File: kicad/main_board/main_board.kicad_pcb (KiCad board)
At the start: 2 copper layers, 42 parts, among them J1 Barrel_Jack, J2 MSTBA 5.08mm 01x02, J3 61400826021, J4 0.1" Male 01x03, J5 0.1" Male 01x03, J6 Conn_ARM_JTAG_SWD_10, Q1 FQP27P06, U2 Pico

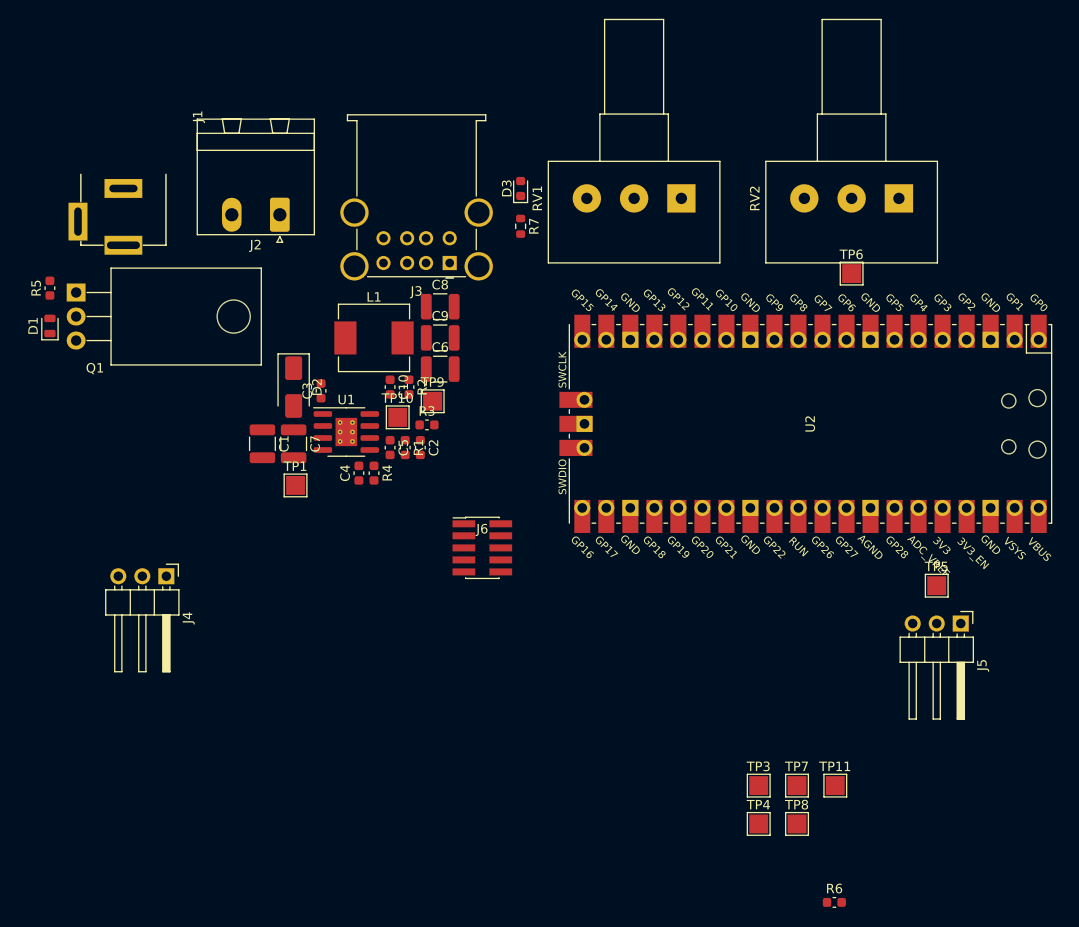
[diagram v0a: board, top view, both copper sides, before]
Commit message: First working version
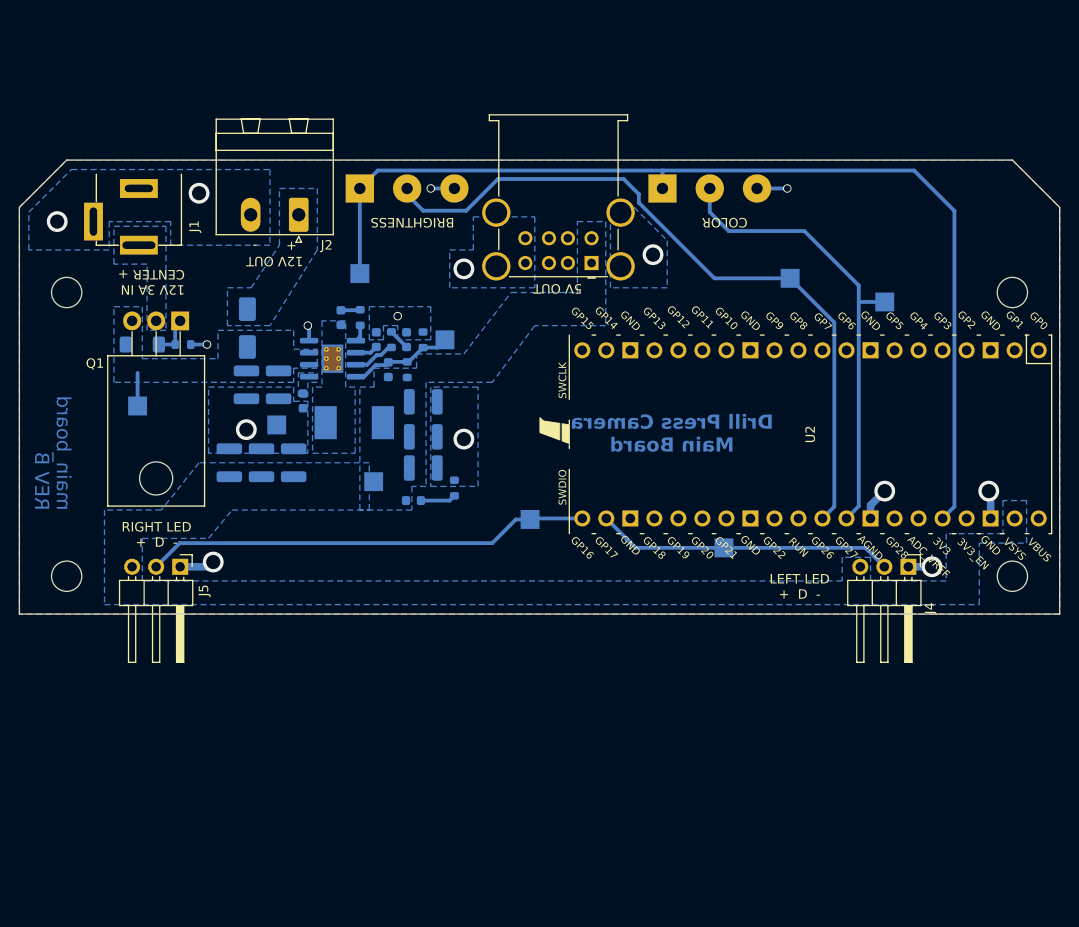
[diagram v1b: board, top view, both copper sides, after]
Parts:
- removed J6: Conn_ARM_JTAG_SWD_10, Connector_PinHeader_1.27mm:PinHeader_2x05_P1.27mm_Vertical_SMD
- removed R6: 10k, Capacitor_SMD:C_0603_1608Metric
- removed TP8: TestPoint, TestPoint:TestPoint_Pad_2.0x2.0mm
- added C11: 22uF X7R 25V, Capacitor_SMD:C_1210_3225Metric, B.Cu at (113.0, 70.0)
- added C12: 22uF X7R 25V, Capacitor_SMD:C_1210_3225Metric, B.Cu at (109.6, 70.0)
- added C13: 22uF X7R 25V, Capacitor_SMD:C_1210_3225Metric, B.Cu at (106.2, 70.0)
- added GRAPHIC1: Graphic, Custom_Graphic:bird_with_pants_small_flipped, F.Cu at (140.6, 66.4)
- added H1: MountingHole, MountingHole:MountingHole_3.2mm_M3, F.Cu at (89.0, 52.0)
- added H2: MountingHole, MountingHole:MountingHole_3.2mm_M3, F.Cu at (189.0, 52.0)
- added H3: MountingHole, MountingHole:MountingHole_3.2mm_M3, F.Cu at (189.0, 82.0)
- added H4: MountingHole, MountingHole:MountingHole_3.2mm_M3, F.Cu at (89.0, 82.0)
- added PCB1: PCB, Custom_Graphic:PCB_PN_REV, B.Cu at (86.0, 66.7)
- C1, C2, C3, C4, C5, C6, C7, C8, C9, D2, D3, L1, R7, RV1, RV2, TP1, TP10, TP11, TP3, TP4, TP5, TP6, TP7, TP9: moved to B.Cu
- C10: value 47pF -> DNP; moved to B.Cu
- D1: footprint Diode_SMD:D_MicroMELF -> Diode_SMD:D_MiniMELF; moved to B.Cu
- R1, R4, R5: footprint Capacitor_SMD:C_0603_1608Metric -> Resistor_SMD:R_0603_1608Metric; moved to B.Cu
- R2: value 15k 1% -> 110k 1%; footprint Capacitor_SMD:C_0603_1608Metric -> Resistor_SMD:R_0603_1608Metric; moved to B.Cu
- R3: value 110k 1% -> 15k 1%; footprint Capacitor_SMD:C_0603_1608Metric -> Resistor_SMD:R_0603_1608Metric; moved to B.Cu
- U1: value ~ -> AOZ6605PI-1; footprint Package_SO:SOIC-8-1EP_3.9x4.9mm_P1.27mm_EP2.29x3mm_ThermalVias -> Custom_Package_SO:SOIC-8-1EP_3.9x4.9mm_P1.27mm_EP2.29x3mm_ThermalVias; moved to B.Cu
- U2: footprint Custom_Module:RPi_Pico_SMD_TH -> Custom_Module:RPi_Pico_TH_Socket
- moved TP11 84.0 mm to (96.5, 64.0), turned to 180 degrees
- moved J5 82.8 mm to (101.0, 81.0)
- moved J4 78.5 mm to (178.0, 81.0)
- moved TP3 68.6 mm to (120.0, 50.0), turned to 180 degrees
- moved TP7 53.6 mm to (165.5, 50.5), turned to 180 degrees
- moved TP5 43.6 mm to (138.0, 76.0), turned to 180 degrees
- moved D3 34.9 mm to (125.7, 74.0), turned to 180 degrees
- moved RV1 34.0 mm to (120.0, 41.0)
- moved TP4 29.4 mm to (158.5, 79.0), turned to 180 degrees
- moved R7 28.5 mm to (130.0, 72.7), turned to 90 degrees
- moved RV2 25.0 mm to (152.0, 41.0)
- moved C8 17.2 mm to (126.7, 70.6)
- moved C4 16.6 mm to (118.0, 54.6), turned to -90 degrees
- moved R4 16.5 mm to (120.0, 54.6), turned to 90 degrees
- moved R5 15.3 mm to (101.3, 57.5), turned to 0 degrees
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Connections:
- J4 pad 1: +5V -> GND
- J4 pad 3: GND -> +5V
- J5 pad 1: +5V -> GND
- J5 pad 3: GND -> +5V
- U2 pad 1: /LED_LEFT_DATA -> unconnected-(U2-GPIO0-Pad1)
- U2 pad 2: /LED_RIGHT_DATA -> unconnected-(U2-GPIO1-Pad2)
- U2 pad 21: unconnected-(U2-GPIO16-Pad21) -> /LED_RIGHT_DATA
- U2 pad 22: unconnected-(U2-GPIO17-Pad22) -> /LED_LEFT_DATA
- U2 pad 30: /~{RESET} -> unconnected-(U2-RUN-Pad30)
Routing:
- net +3V3: track 0.00 -> 109.4 mm
- net /BRIGHTNESS_CTRL: track 0.00 -> 76.0 mm
- net /COLOR_CTRL: track 0.00 -> 49.4 mm
- net /LED_RIGHT_DATA: track 0.00 -> 47.2 mm
- net /LED_LEFT_DATA: track 0.00 -> 31.5 mm
- net GND: track 0.00 -> 22.1 mm, vias 0 -> 15
- net /BUCK_FB: track 0.00 -> 11.0 mm
- net Net-(U1-COMP): track 0.00 -> 4.51 mm
- net Net-(D1-A): track 0.00 -> 4.44 mm
- net Net-(D3-K): track 0.00 -> 3.75 mm
- net +12V: track 0.00 -> 3.50 mm
- net Net-(U1-VCC): track 0.00 -> 2.41 mm
- net Net-(C2-Pad1): track 0.00 -> 2.26 mm
- net Net-(C4-Pad1): track 0.00 -> 2.06 mm
- net Net-(U1-BST): track 0.00 -> 1.81 mm
- added copper zone on B.Cu, net +12V
- added copper zone on B.Cu, net +5V
- added copper zone on B.Cu, net GND
- added copper zone on F.Cu, net GND
- added copper zone on B.Cu, net Net-(D2-K)
- added copper zone on B.Cu, net Net-(Q1-D)
- added copper zone on B.Cu, net Net-(U1-LX)
- added copper zone on B.Cu, net Net-(U1-SS)
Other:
- board outline added: 110 x 48 mm
- board text added: "12V 3A IN CENTER +"
- board text added: "12V OUT + -"
- board text added: "5V OUT"
- board text added: "BRIGHTNESS"
- board text added: "COLOR"
- board text added: "Drill Press Camera Main Board"
- board text added: "LEFT LED + D -"
- board text added: "RIGHT LED + D -"
